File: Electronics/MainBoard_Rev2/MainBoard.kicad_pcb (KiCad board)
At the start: 2 copper layers, 57.2 x 35.1 mm, 70 parts, among them J1 Conn_01x04_Female, J2 DB9_Female, J3 USB_B_Micro, J4 Conn_01x04_Male, J5 Conn_01x02_Male, Q30 PMBT2222A, Q35 PMBT2222A, Q5 Q_NPN_BEC, Q6 Q_NPN_BEC, U1 ESP32-WROOM-32, U13 FT231XS, U3 LSM6DS3, U4 MAX1555EZK_T, U50 AP2114H-3_3TRG1

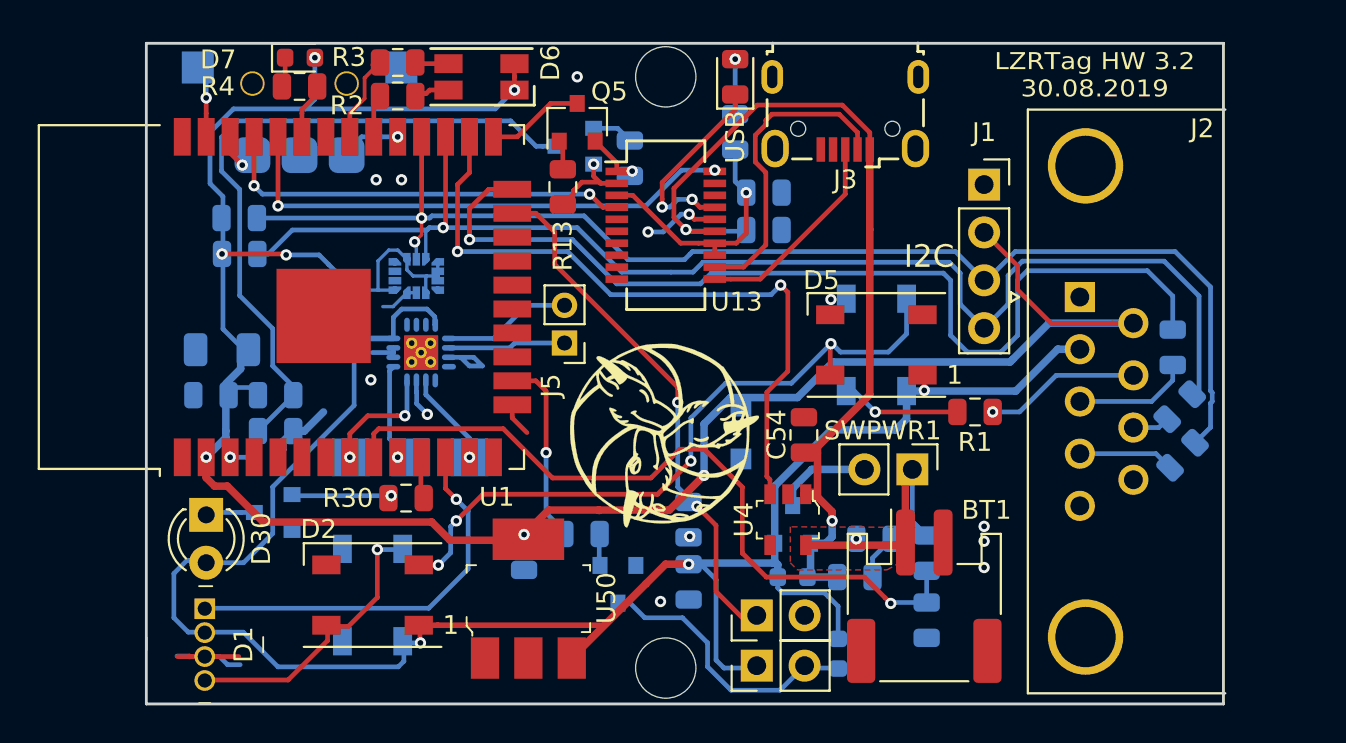
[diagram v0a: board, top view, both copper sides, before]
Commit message: Modify board for the v3.3 release-ish
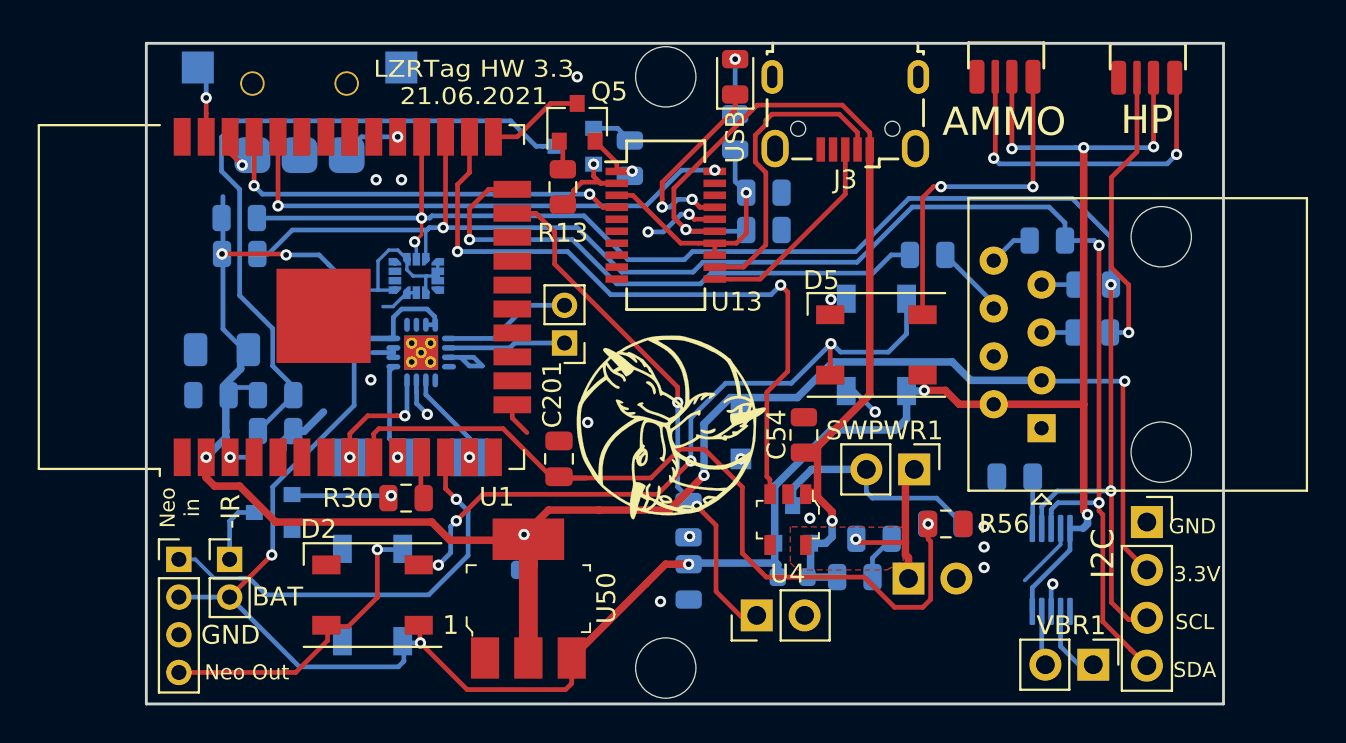
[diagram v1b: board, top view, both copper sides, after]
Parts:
- removed D35: D_Schottky, Diode_SMD:D_0603_1608Metric
- removed D6: LED_Dual_AACC, LED_SMD:LED_RGB_1210
- removed D7: LED, LED_SMD:LED_0603_1608Metric
- removed J2: DB9_Female, Connector_Dsub:DSUB-9_Female_Horizontal_P2.77x2.84mm_EdgePinOffset4.94mm_Housed_MountingHolesOffset7.48mm
- removed Q35: PMBT2222A, Package_TO_SOT_SMD:SOT-23
- removed R2, R3: 220R, Resistor_SMD:R_0805_2012Metric
- removed R35: 2.2k, Resistor_SMD:R_0805_2012Metric
- removed R4: 220, Resistor_SMD:R_0805_2012Metric
- added C201: 0.1uF, Capacitor_SMD:C_0805_2012Metric, F.Cu at (85.4, 101.3)
- added C401: 1uF, Capacitor_SMD:C_0805_2012Metric, B.Cu at (109.6, 102.3)
- added D401: IN-PI42TAS, XasPrints:IN-PI42TAS, F.Cu at (109.1, 80.8)
- added D402: IN-PI42TAS, XasPrints:IN-PI42TAS, F.Cu at (116.6, 80.9)
- added J101: 54602-908LF, Connector_RJ:RJ45_Amphenol_54602-x08_Horizontal, F.Cu at (111.0, 99.7)
- added U401: DRV2605, Package_SO:VSSOP-10_3x3mm_P0.5mm, B.Cu at (111.5, 107.2)
- BT1: footprint Connector_JST:JST_PH_S2B-PH-SM4-TB_1x02-1MP_P2.00mm_Horizontal -> Connector_PinHeader_2.54mm:PinHeader_1x02_P2.54mm_Horizontal; moved to B.Cu
- C2, C31, C8: value 150nF -> 100nF
- C3: value 0.1uF -> 100nF
- D1: footprint digikey-footprints:LED_RGB_WP154A4SUREQBFZGC -> Connector_PinHeader_2.00mm:PinHeader_1x04_P2.00mm_Vertical
- D30: value SFH4346 -> SFH4545; footprint LED_THT:LED_D3.0mm_IRBlack -> Connector_PinHeader_2.00mm:PinHeader_1x02_P2.00mm_Vertical
- R1: value 220 -> 220R; moved to B.Cu
- R13, R14: value R_Small -> 10k
- R30, R7, R8, R9: value 220 -> 220R
- R55: value 100k -> 50k
- R56: value 200k -> 50k; moved to F.Cu
- U3: value LSM6DS3 -> LSM6DSMTR
- moved H4 27.5 mm to (100.6, 83.9), turned to 0 degrees
- moved H3 22.2 mm to (87.4, 103.5)
- moved J1 19.9 mm to (116.6, 104.6)
- moved VBR1 17.9 mm to (113.7, 112.2), turned to 270 degrees
- moved R7 13.9 mm to (105.0, 90.5), turned to 180 degrees
- moved R8 11.3 mm to (111.3, 89.7), turned to 0 degrees
- moved R9 10.2 mm to (113.7, 92.0), turned to 0 degrees
- moved R1 7.52 mm to (113.7, 94.6), turned to 0 degrees
- moved R56 5.21 mm to (105.9, 104.7), turned to 0 degrees
- moved D1 4.72 mm to (65.2, 106.6), turned to 0 degrees
- moved D30 2.67 mm to (67.9, 106.6), turned to 0 degrees
- moved R55 1.83 mm to (105.9, 104.7), turned to 180 degrees
- moved BT1 1.26 mm to (103.9, 107.6), turned to 270 degrees
- moved H6 0.56 mm to (91.1, 99.5)
- moved SWPWR1 0.10 mm to (104.2, 101.9)
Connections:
- AMP1 pad 7: Net-(AMP1-Pad7) -> +BATT
- BT1 pad 1: /PowerHandling/B_Raw+ -> Net-(BT1-Pad1)
- C53 pad 1: /PowerHandling/B_Raw+ -> Net-(BT1-Pad1)
- D4 pad 2: /LED_2 -> Net-(D4-Pad2)
- QPWR1 pad 3: Net-(QPWR1-Pad3) -> /PowerHandling/B_Raw+
- SWPWR1 pad 1: /PowerHandling/B_Raw+ -> Net-(BT1-Pad1)
- SWPWR1 pad 2: Net-(QPWR1-Pad3) -> /PowerHandling/B_Raw+
- U1 pad 16: /VBRT -> Net-(U1-Pad16)
- U1 pad 30: /CHG_R -> Net-(U1-Pad30)
- U1 pad 31: /CHG_G -> Net-(U1-Pad31)
- U1 pad 33: /CONN_IND -> Net-(U1-Pad33)
- U1 pad 39: (no net) -> GND
- U4 pad 5: /PowerHandling/B_Raw+ -> Net-(BT1-Pad1)
- U50 pad 2: Net-(U50-Pad2) -> +3V3
- VBR1 pad 1: +BATT -> Net-(U401-Pad7)
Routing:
- net +BATT: track 106.8 -> 130.8 mm, vias 3 -> 8
- net /IR_IN: track 52.1 -> 29.3 mm
- net +3V3: track 129.1 -> 109.3 mm, vias 7 -> 6
- net Net-(D401-Pad2): track 0.00 -> 18.5 mm, vias 0 -> 2
- net Net-(D401-Pad4): track 0.00 -> 18.1 mm, vias 0 -> 2
- net SDA: track 69.0 -> 82.5 mm, vias 1 -> 3
- net SCL: track 69.3 -> 82.2 mm, vias 2 -> 4
- net Net-(U401-Pad9): track 14.8 -> 2.91 mm
- net /VBRT: track 10.2 -> 0.00 mm, vias 1 -> 0
- net /LED_2: track 6.35 -> 15.4 mm
- net Net-(BT1-Pad1): track 0.00 -> 8.76 mm, vias 0 -> 1
- net Net-(J101-Pad5): track 8.27 -> 1.75 mm, vias 1 -> 0
- net /V_SENSE: track 39.6 -> 44.8 mm
- net /CHG_G: track 5.15 -> 0.00 mm
- net Net-(QPWR1-Pad3): track 5.14 -> 0.00 mm
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- added copper zone on F.Cu, net Net-(BT1-Pad1)
- removed copper zone on F.Cu, net /PowerHandling/B_Raw+
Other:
- board text added: "-IR"
- board text added: "AMMO"
- board text added: "BAT"
- board text added: "HP"
- board text added: "LZRTag HW 3.3 21.06.2021"
- board text added: "Neo Out"
- board text added: "Neo in"
- board text removed: "LZRTag HW 3.2 30.08.2019"
